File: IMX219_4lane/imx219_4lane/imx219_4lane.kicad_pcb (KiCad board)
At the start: 4 copper layers, 25 x 24 mm, 26 parts, among them J1 DF37NC-30DS-0.4V, J2 FPC 28 pin connector, Q1 NTR5103N, Q2 NTR5103N, U1 AMPM, U2 LM3670MF, U3 AP7331, U4 AP7331

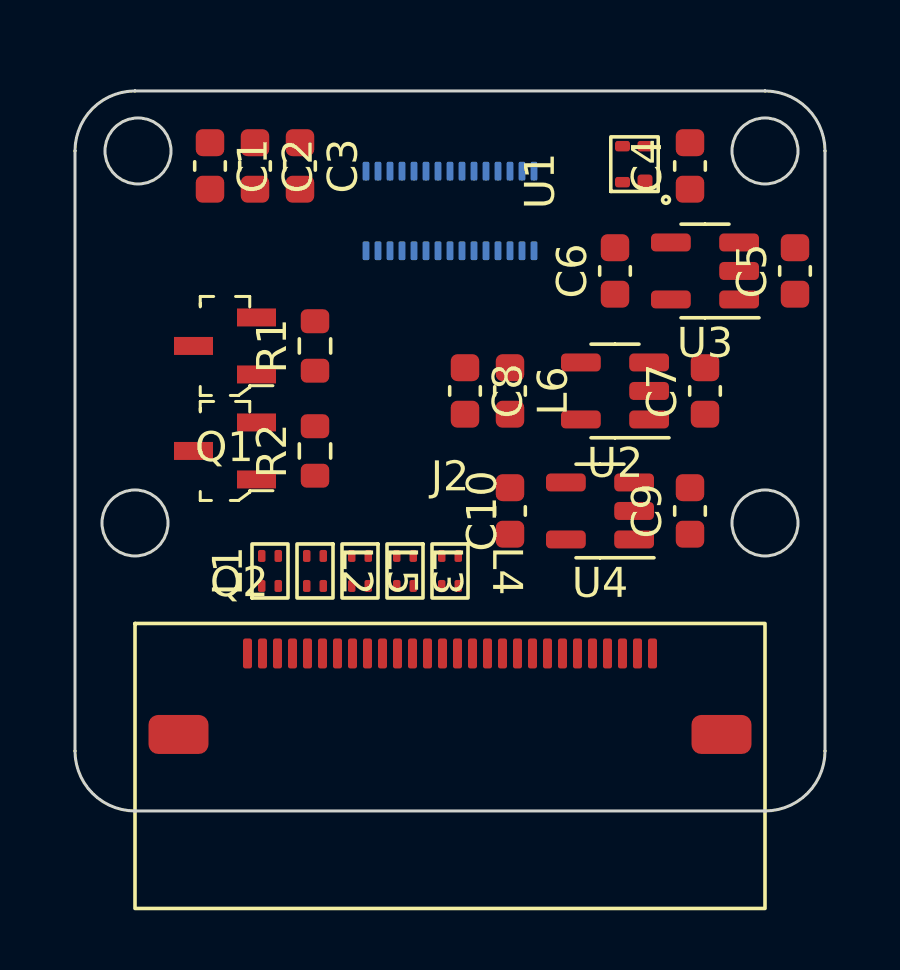
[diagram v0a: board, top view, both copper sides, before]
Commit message: update
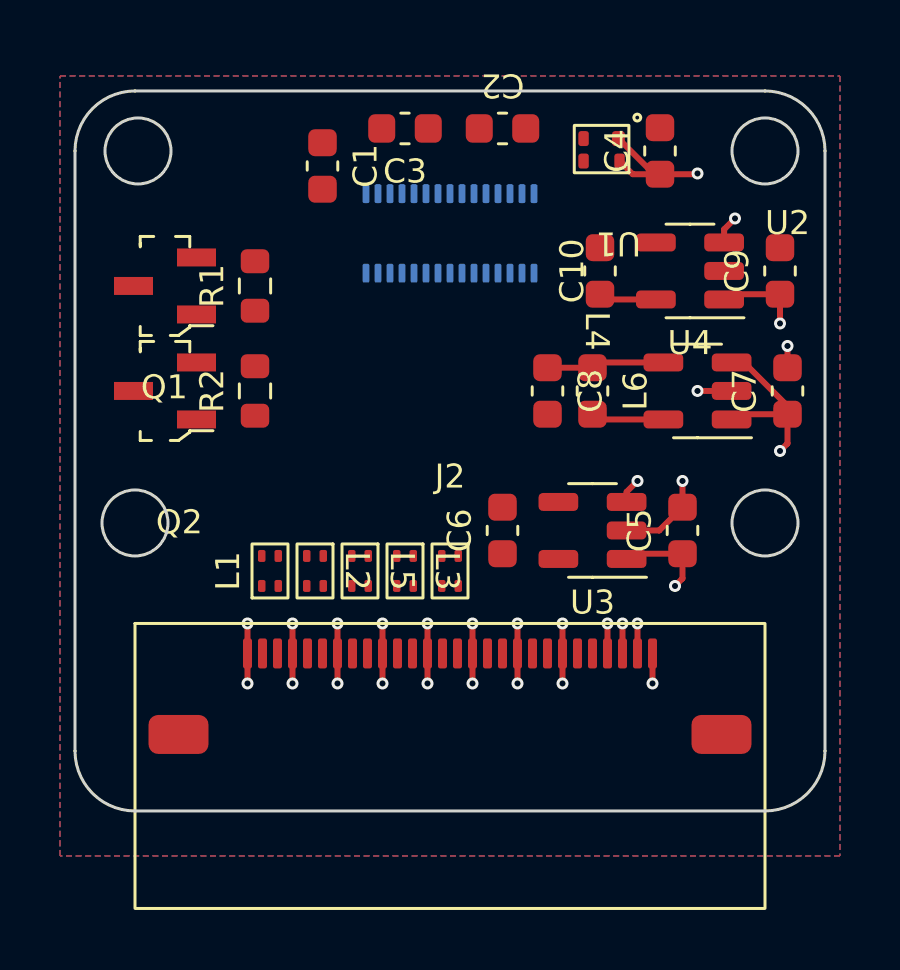
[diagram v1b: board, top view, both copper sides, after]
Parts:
- moved C5 9.43 mm to (40.2, 34.6)
- moved C6 9.43 mm to (34.2, 34.6)
- moved U3 9.43 mm to (37.2, 34.6)
- moved C10 8.54 mm to (37.5, 26.0)
- moved C9 8.54 mm to (43.5, 26.0)
- moved U4 8.54 mm to (40.5, 26.0)
- moved C2 8.34 mm to (34.2, 21.2), turned to 0 degrees
- moved C1 3.75 mm to (28.2, 22.5)
- moved C3 3.72 mm to (31.0, 21.2), turned to 180 degrees
- moved Q1 2.83 mm to (23.0, 26.5)
- moved Q2 2.83 mm to (23.0, 30.0)
- moved R1 2.83 mm to (26.0, 26.5)
- moved R2 2.83 mm to (26.0, 30.0)
- moved C7 2.75 mm to (43.8, 30.0)
- moved C8 2.75 mm to (35.8, 30.0)
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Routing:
- net GND: track 0.00 -> 21.9 mm, vias 0 -> 20
- net +5V: track 0.00 -> 16.8 mm, vias 0 -> 8
- net +1V8: track 0.00 -> 4.67 mm, vias 0 -> 1
- net +1V2: track 0.00 -> 3.93 mm
- net Net-(L6-Pad2): track 0.00 -> 2.43 mm
- net +2V8: track 0.00 -> 1.93 mm
- added copper zone on In1.Cu, net +1V8
- added copper zone on In2.Cu, net +1V8
- added copper zone on In1.Cu, net +5V
- added copper zone on In2.Cu, net +5V
- added copper zone on B.Cu, net GND
- added copper zone on F.Cu, net GND
